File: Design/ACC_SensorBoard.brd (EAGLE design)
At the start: 23.3 x 24.5 mm, 12 parts, among them U2 ADXL345

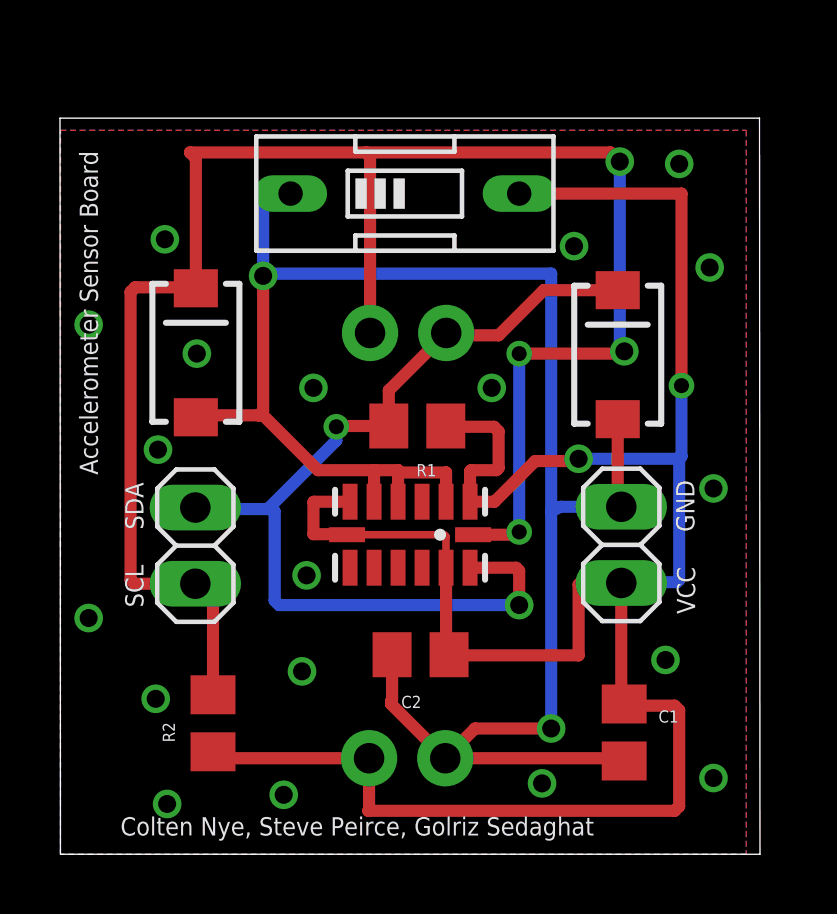
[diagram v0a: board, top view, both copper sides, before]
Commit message: Updating/Cleaning-up documents
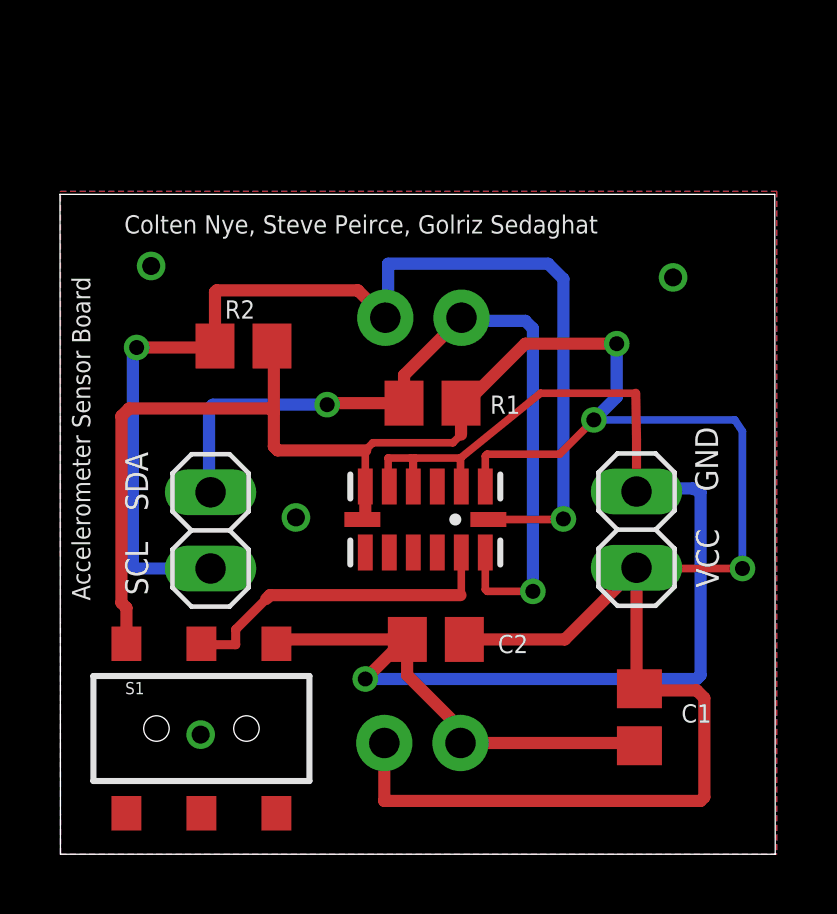
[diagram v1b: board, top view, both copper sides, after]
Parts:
- removed GND, U$1: TVS, SparkFun-DiscreteSemi:SMA-DIODE
- removed SW1: (no value), special:EDG-01
- added S1: (no value), SparkFun-Electromechanical:AYZ0202
- moved R2 12.6 mm to (6.10, 16.9), turned to 180 degrees
- moved R1 0.92 mm to (12.4, 15.0)
- moved C1 0.72 mm to (19.3, 4.57)
- moved F1 0.72 mm to (13.4, 17.9)
- moved F2 0.72 mm to (13.3, 3.71)
- moved U2 0.72 mm to (12.2, 11.2)
- moved C2 0.72 mm to (12.5, 7.16)
- moved M1 0.72 mm to (5.00, 10.8)
- moved M2 0.72 mm to (19.2, 10.8)
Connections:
- new net N$1: S1.2, U2.12
- net +3V3: now also S1.1; no longer SW1.2, U2.12
- net GND: now also S1.3; no longer GND.A, SW1.1, U$1.A
- net SCL_ACC: no longer GND.C
- net SDA_ACC: no longer U$1.C
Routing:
- net SCL_ACC: track 60.6 -> 38.9 mm, vias 4 -> 2
- net GND: track 64.9 -> 52.1 mm, vias 20 -> 5
- net N$1: track 0.00 -> 11.1 mm
- net SDA_ACC: track 32.4 -> 27.2 mm
- net +3V3: track 78.5 -> 83.4 mm, vias 2 -> 3
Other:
- board size 23.3 x 24.5 mm -> 23.8 x 22 mm
